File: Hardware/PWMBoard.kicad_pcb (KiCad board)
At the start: 2 copper layers, 53.3 x 94 mm, 31 parts, among them J1 Screw_Terminal_01x03, J2 Screw_Terminal_01x02, J3 AVR-ISP-6, Q1 IRF540N, Q2 IRF540N, Q3 IRF9540N, Q4 IRF9540N, Q5 BC547, Q6 BC547, U1 ATtiny2313-20P, U2 LM7805_TO220

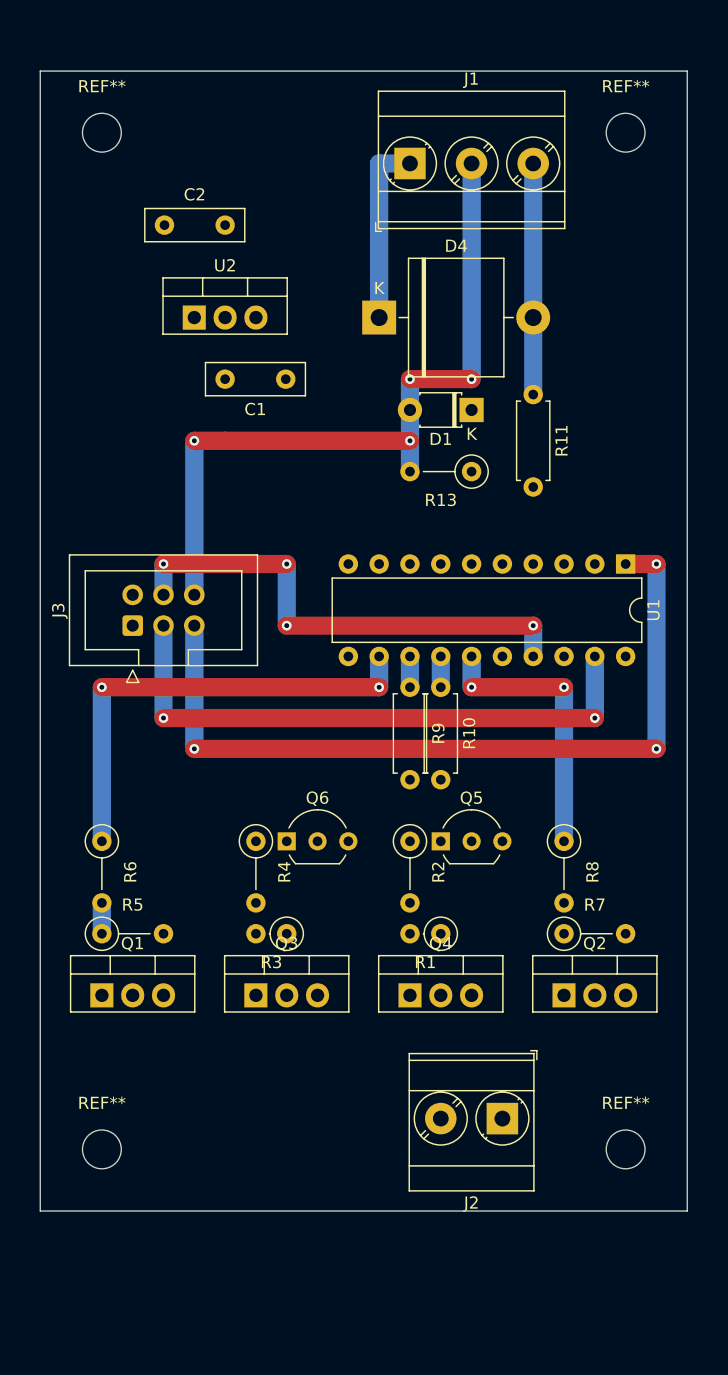
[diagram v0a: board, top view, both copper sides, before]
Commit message: Update PCB
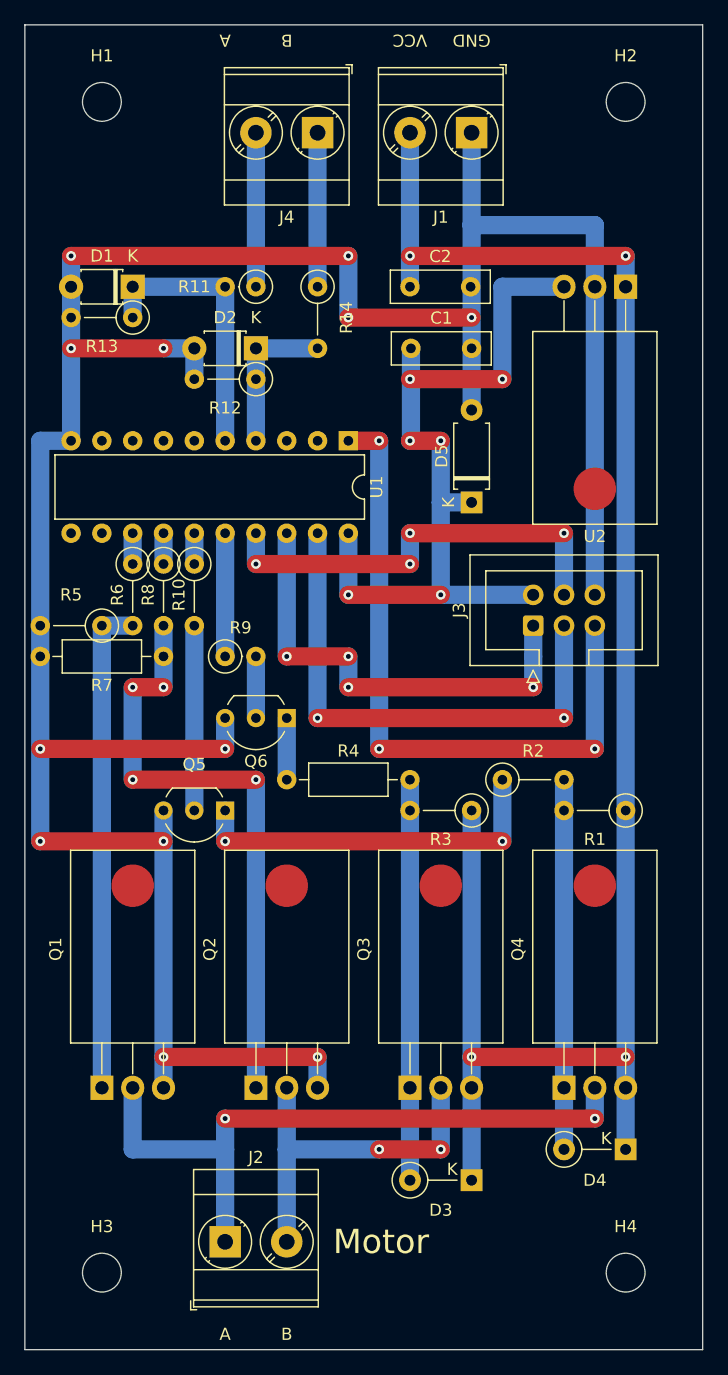
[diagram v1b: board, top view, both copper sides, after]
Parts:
- removed REF** (x4): MountingHole_3.2mm_M3_DIN965, MountingHole:MountingHole_3.2mm_M3_DIN965
- added D2: 4.7V, Diode_THT:D_T-1_P5.08mm_Horizontal, F.Cu at (94.0, 73.7)
- added D3: 12V, Diode_THT:D_A-405_P5.08mm_Vertical_KathodeUp, F.Cu at (111.8, 142.2)
- added D5: 5V1, Diode_THT:D_A-405_P7.62mm_Horizontal, F.Cu at (111.8, 86.4)
- added H1: MountingHole, MountingHole:MountingHole_3.2mm_M3_DIN965, F.Cu at (81.3, 53.3)
- added H2: MountingHole, MountingHole:MountingHole_3.2mm_M3_DIN965, F.Cu at (124.5, 53.3)
- added H3: MountingHole, MountingHole:MountingHole_3.2mm_M3_DIN965, F.Cu at (81.3, 149.9)
- added H4: MountingHole, MountingHole:MountingHole_3.2mm_M3_DIN965, F.Cu at (124.5, 149.9)
- added J4: Screw_Terminal_01x02, TerminalBlock_Phoenix:TerminalBlock_Phoenix_MKDS-3-2-5.08_1x02_P5.08mm_Horizontal, F.Cu at (99.1, 55.9)
- added R12: 10k, Resistor_THT:R_Axial_DIN0207_L6.3mm_D2.5mm_P5.08mm_Vertical, F.Cu at (94.0, 76.2)
- added R14: 10k, Resistor_THT:R_Axial_DIN0207_L6.3mm_D2.5mm_P5.08mm_Vertical, F.Cu at (99.1, 68.6)
- D4: value D_Schottky -> 12V; footprint Diode_THT:D_5KP_P12.70mm_Horizontal -> Diode_THT:D_A-405_P5.08mm_Vertical_KathodeUp
- J1: value Screw_Terminal_01x03 -> Screw_Terminal_01x02; footprint TerminalBlock_Phoenix:TerminalBlock_Phoenix_MKDS-3-3-5.08_1x03_P5.08mm_Horizontal -> TerminalBlock_Phoenix:TerminalBlock_Phoenix_MKDS-3-2-5.08_1x02_P5.08mm_Horizontal
- Q1, Q2, Q3, Q4, U2: footprint Package_TO_SOT_THT:TO-220-3_Vertical -> Package_TO_SOT_THT:TO-220-3_Horizontal_TabDown
- R1, R3: footprint Resistor_THT:R_Axial_DIN0207_L6.3mm_D2.5mm_P2.54mm_Vertical -> Resistor_THT:R_Axial_DIN0207_L6.3mm_D2.5mm_P5.08mm_Vertical
- R10: footprint Resistor_THT:R_Axial_DIN0207_L6.3mm_D2.5mm_P7.62mm_Horizontal -> Resistor_THT:R_Axial_DIN0207_L6.3mm_D2.5mm_P5.08mm_Vertical
- R11, R9: footprint Resistor_THT:R_Axial_DIN0207_L6.3mm_D2.5mm_P7.62mm_Horizontal -> Resistor_THT:R_Axial_DIN0207_L6.3mm_D2.5mm_P2.54mm_Vertical
- R13: value 100k -> 10k
- R4: footprint Resistor_THT:R_Axial_DIN0207_L6.3mm_D2.5mm_P5.08mm_Vertical -> Resistor_THT:R_Axial_DIN0207_L6.3mm_D2.5mm_P10.16mm_Horizontal
- R5: value 2.2k -> 10k
- R7: value 2.2k -> 10k; footprint Resistor_THT:R_Axial_DIN0207_L6.3mm_D2.5mm_P5.08mm_Vertical -> Resistor_THT:R_Axial_DIN0207_L6.3mm_D2.5mm_P10.16mm_Horizontal
- moved D4 71.5 mm to (124.5, 139.7), turned to 180 degrees
- moved R7 40.2 mm to (86.4, 99.1), turned to 180 degrees
- moved R8 40.2 mm to (86.4, 91.4)
- moved U2 35.7 mm to (124.5, 68.6), turned to 180 degrees
- moved J3 33.0 mm to (116.8, 96.5)
- moved R13 30.7 mm to (83.8, 71.1)
- moved D1 29.7 mm to (83.8, 68.6)
- moved Q2 26.5 mm to (94.0, 134.6)
- moved R5 25.4 mm to (81.3, 96.5), turned to 180 degrees
- moved J2 25.0 mm to (91.4, 147.3), turned to 0 degrees
- moved U1 25.0 mm to (101.6, 81.3)
- moved R11 24.5 mm to (94.0, 68.6), turned to 180 degrees
- moved R6 23.0 mm to (83.8, 91.4)
- moved R10 22.7 mm to (88.9, 91.4)
- moved C2 20.9 mm to (106.7, 68.6)
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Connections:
- D1 pad 1: /cDown -> /a
- D4 pad 2: /down -> /AH
- J1 pad 1: VCC -> GND
- J1 pad 2: GND -> VCC
- J2 pad 1: /A -> /motorA
- J2 pad 2: /B -> /motorB
- Q1 pad 2: /A -> /motorA
- Q2 pad 2: /B -> /motorB
- Q3 pad 2: VCC -> /motorB
- Q3 pad 3: /B -> VCC
- Q4 pad 2: VCC -> /motorA
- Q4 pad 3: /A -> VCC
- R11 pad 1: /down -> /A
- R11 pad 2: /cDown -> /a
- R13 pad 1: /cDown -> /a
- U1 pad 12: /cAL -> unconnected-(U1-PB0-Pad12)
- U1 pad 13: /cBH -> /cAL
- U1 pad 14: /cAH -> /cBL
- U1 pad 15: /cBL -> /cAH
- U1 pad 16: unconnected-(U1-PB4-Pad16) -> /cBH
- U1 pad 4: unconnected-(U1-PA1/XTAL2-Pad4) -> /b
- U1 pad 5: unconnected-(U1-PA0/XTAL1-Pad5) -> /a
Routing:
- net GND: track 61.0 -> 231.1 mm, vias 4 -> 12
- net VCC: track 15.2 -> 147.3 mm, vias 0 -> 4
- net +5V: track 0.00 -> 66.1 mm, vias 0 -> 6
- net /motorA: track 0.00 -> 55.9 mm, vias 0 -> 2
- net /BL: track 0.00 -> 50.8 mm, vias 0 -> 4
- net /miso: track 0.00 -> 38.1 mm, vias 0 -> 4
- net /AL: track 2.54 -> 40.6 mm
- net /cAL: track 38.1 -> 2.54 mm, vias 2 -> 0
- net /BH: track 0.00 -> 33.0 mm
- net Net-(Q5-C): track 0.00 -> 30.5 mm, vias 0 -> 2
- net /AH: track 0.00 -> 30.5 mm
- net /motorB: track 0.00 -> 30.5 mm, vias 0 -> 2
- net /a: track 0.00 -> 22.9 mm
- net /cBL: track 22.9 -> 2.54 mm, vias 2 -> 0
- net /down: track 19.0 -> 0.00 mm
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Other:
- board size 53.3 x 94 mm -> 55.9 x 109.2 mm
- board text added: "A"
- board text added: "B"
- board text added: "GND"
- board text added: "Motor"
- board text added: "VCC"
